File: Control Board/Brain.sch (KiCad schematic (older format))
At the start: 36 parts, among them J10 USB_B_Micro, J11 Conn_ARM_JTAG_SWD_10, J9 Conn_ARM_JTAG_SWD_10, SW2 SW_Push, U1 ATSAMD21G18A-AU, U6 AT24C32, Y1 32768Hz

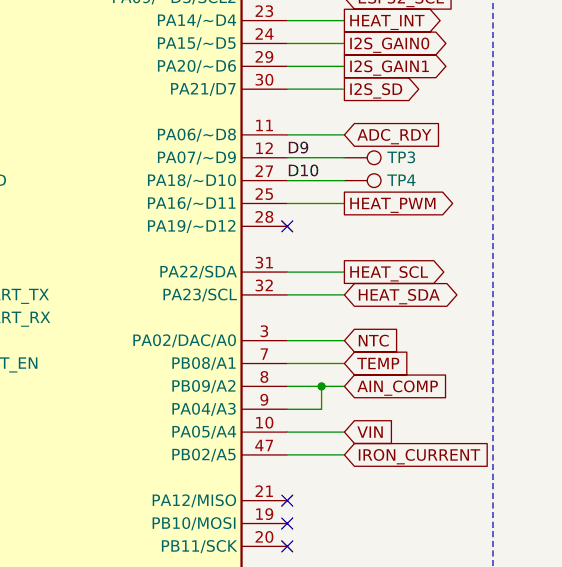
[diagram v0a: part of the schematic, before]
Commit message: More erratum.
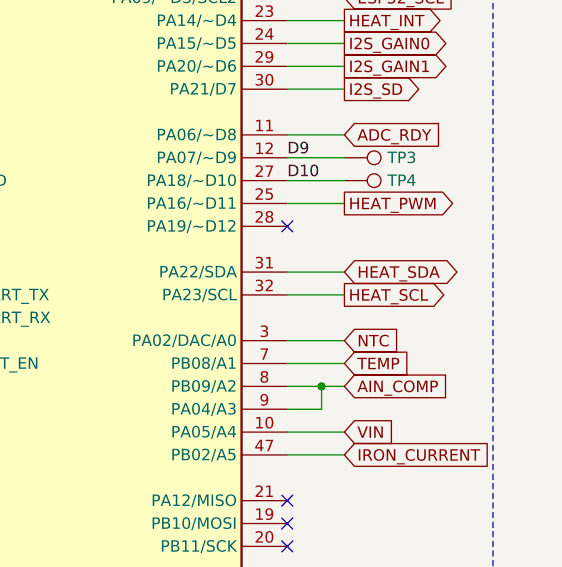
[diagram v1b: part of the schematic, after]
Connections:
- net HEAT_SCL: now also U1.32 (PA23/SCL); no longer U1.31 (PA22/SDA)
- net HEAT_SDA: now also U1.31 (PA22/SDA); no longer U1.32 (PA23/SCL)
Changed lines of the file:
@@
 Sheet 4 5
 Title "IoT12-hardware brain"
-Date "2021-03-12"
+Date "2021-03-13"
 Rev "V2.1"
 Comp ""
@@
 	1    0    0    -1
 $EndComp
-Text GLabel 10500 3200 2    50   Output ~ 0
+Text GLabel 10500 3300 2    50   Output ~ 0
 HEAT_SCL
 Wire Wire Line
-	10500 3200 10250 3200
-Text GLabel 10500 3300 2    50   BiDi ~ 0
+	10500 3300 10250 3300
+Text GLabel 10500 3200 2    50   BiDi ~ 0
 HEAT_SDA
 $Comp
@@
 	11150 5200 11150 550
 Wire Wire Line
-	10500 3300 10250 3300
+	10500 3200 10250 3200
 Wire Wire Line
 	7850 1600 8250 1600
